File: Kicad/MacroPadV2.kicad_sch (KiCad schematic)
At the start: 63 parts, among them J1 3PinJump, J2 3PinJump, J3 GCT-USB4085, J4 3PinJump, J5 4PinJump, J6 4PinJump, J7 4PinJump, K1 KSW, K10 KSW, K11 KSW, K12 KSW, K2 KSW, K3 KSW, K4 KSW, K5 KSW, K6 KSW, K7 KSW, K8 KSW, K9 KSW, SW1 SWITCH_TACTILE_SPST-NO_0.05A_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, SW2 SWITCH_TACTILE_SPST-NO_0.05A_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, SW3 RotaryEncoder_Switch, U1 STM32F103C8T6TR, U2 AP2114HA-3.3TRG1, X1 TSX-3225_16.0000MF18X-AC6

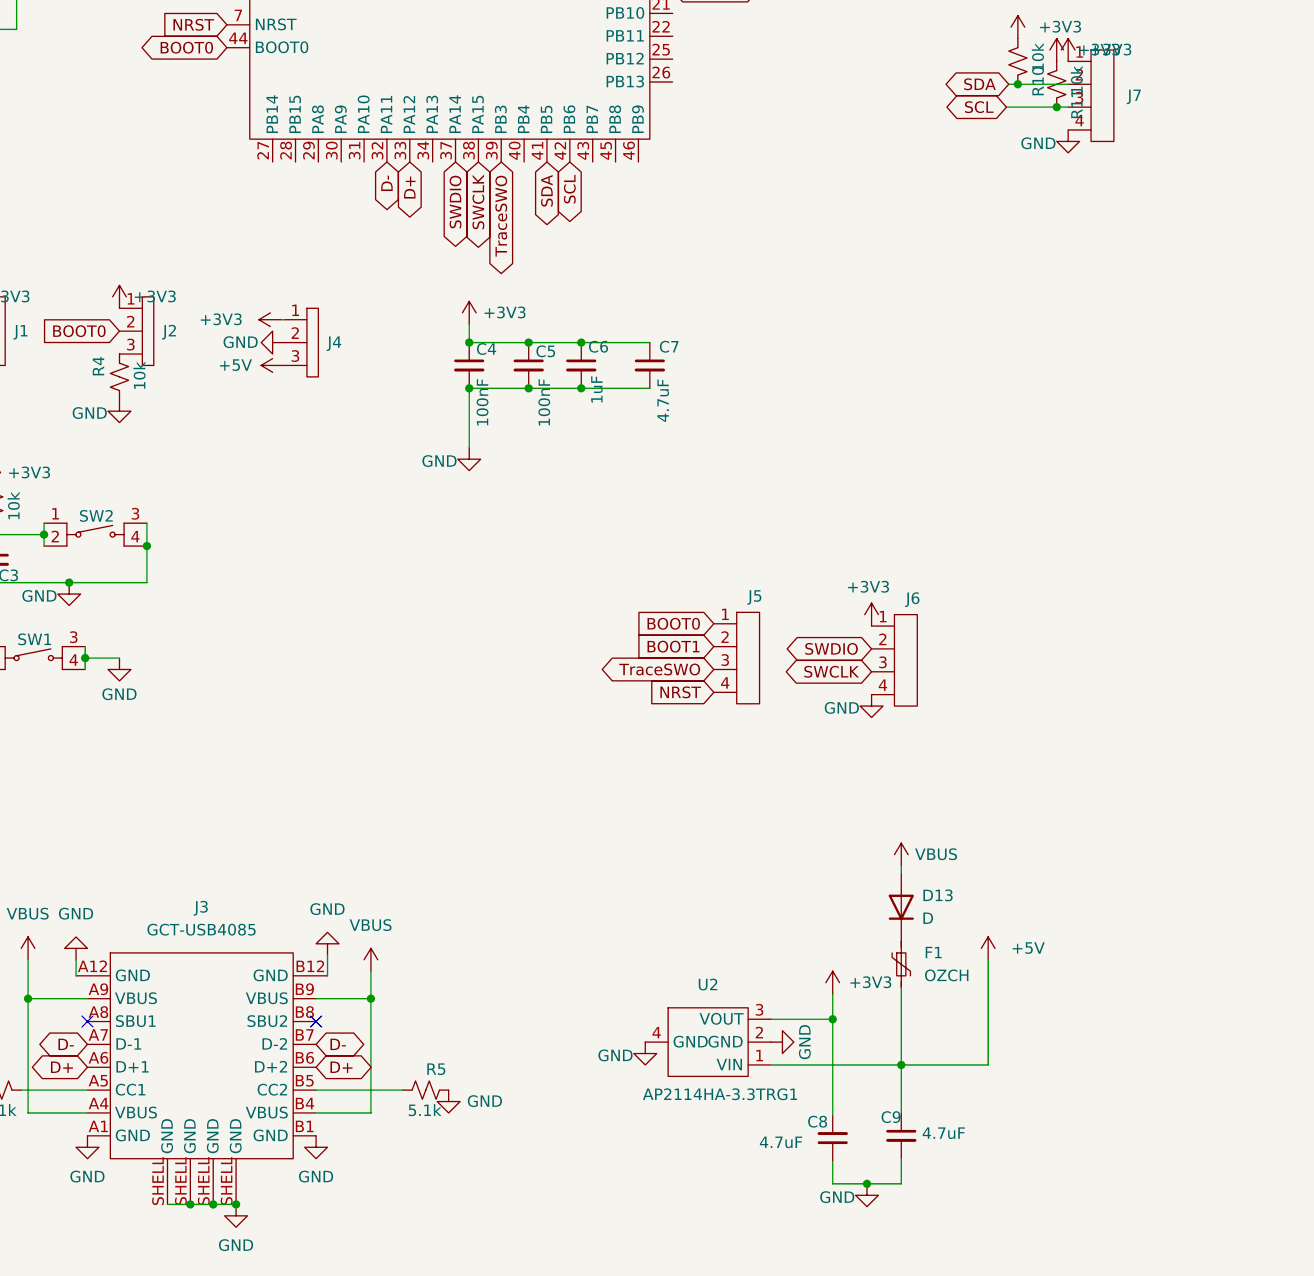
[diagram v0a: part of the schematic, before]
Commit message: Removed some backups and push for swap to desktop
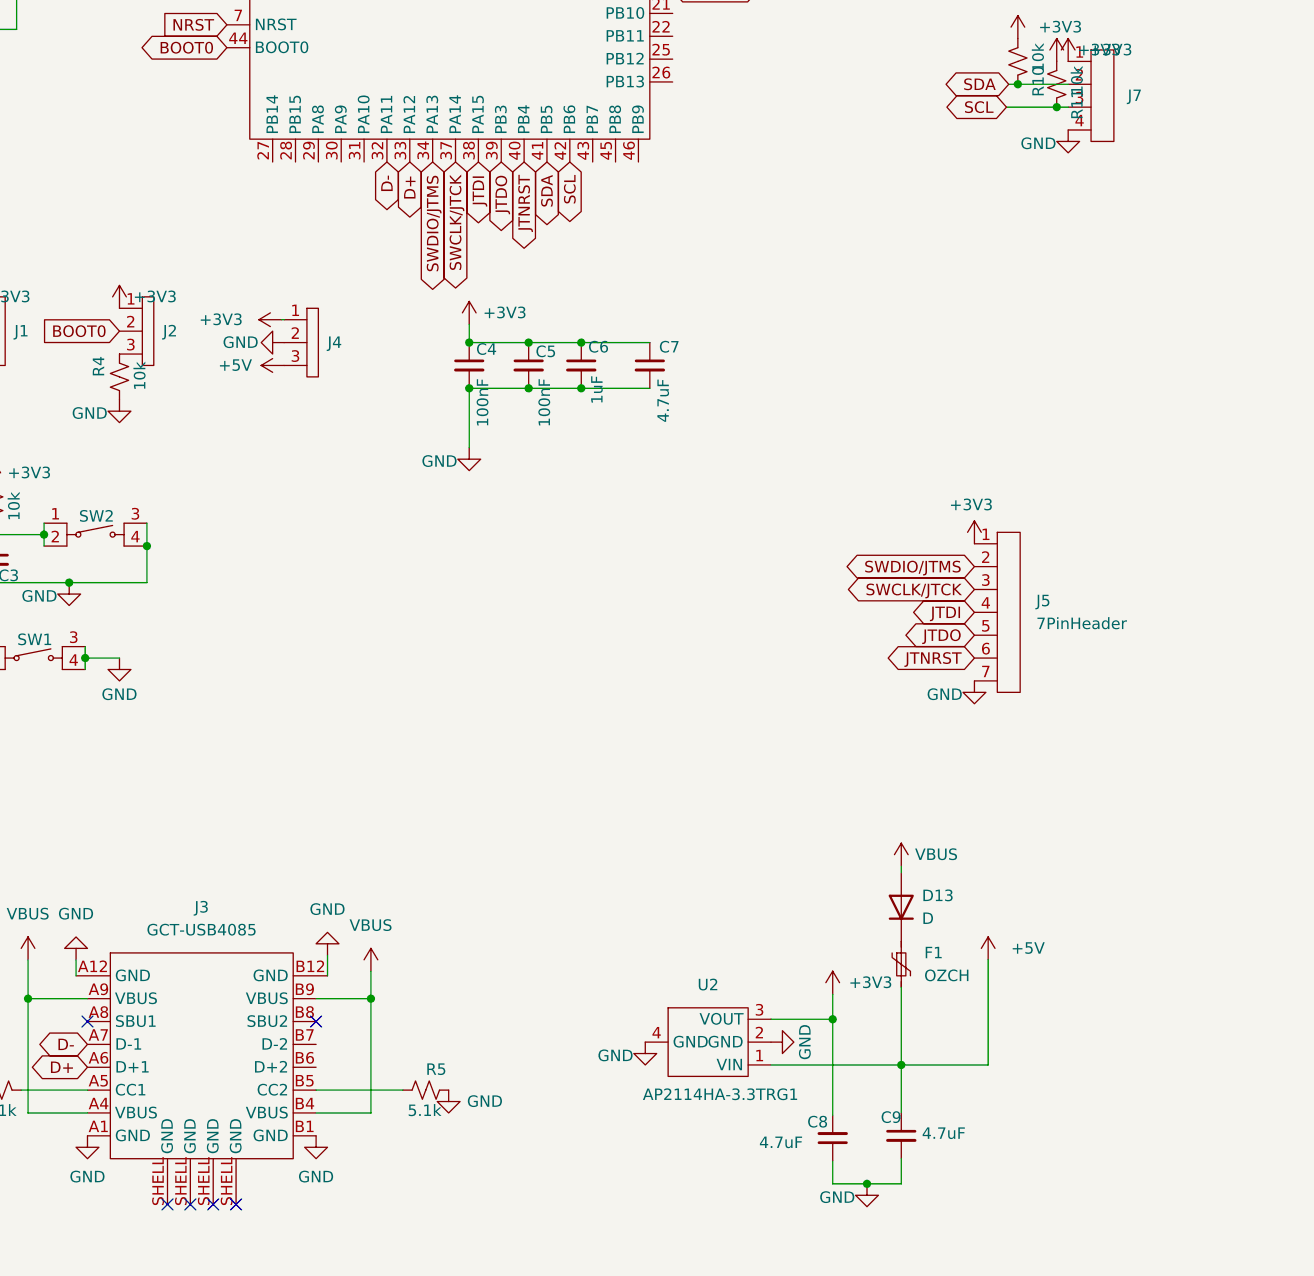
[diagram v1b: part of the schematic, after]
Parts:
- removed J5, J6: 4PinJump, Connector_PinHeader_2.54mm:PinHeader_1x04_P2.54mm_Vertical, symbol macropad_parts:4PinJump
- added J5: 7PinHeader, Connector_PinHeader_2.54mm:PinHeader_1x07_P2.54mm_Vertical, symbol macropad_parts:7PinHeader
- U1: footprint macrofp:LQFP48 -> mpadfps:LQFP48
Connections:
- net +3V3: now also J5.1
- net D+: no longer J3.B6 (D+2)
- net D-: no longer J3.B7 (D-2)
- net GND: now also J5.7; no longer J3.SHELL (GND)
- net SWDIO/JTMS: now reaches U1.34 (PA13)
- net SWDIO/JTMS: now also J5.2
- net JTNRST: now reaches U1.40 (PB4)
- net JTNRST: now also J5.6
- net SWCLK renamed JTDI
- net JTDI: now also J5.4
- net SWDIO renamed SWCLK/JTCK
- net SWCLK/JTCK: now also J5.3
- net TraceSWO renamed JTDO
- net JTDO: now also J5.5
- no-connect marks 2 -> 6
